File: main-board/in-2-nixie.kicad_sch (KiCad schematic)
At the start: 33 parts, among them J1 Encoder, J2 Matrix, J3 Buttons, J4 Power, J5 BME280, J6 DS3231, Q1 MPSA42, T1 IN-2, T2 IN-2, T3 IN-2, T4 IN-2, U1 HV5222PJ, U2 Nixie HVPS, U3 ESP32-C6 SuperMini, U4 Level Shifter

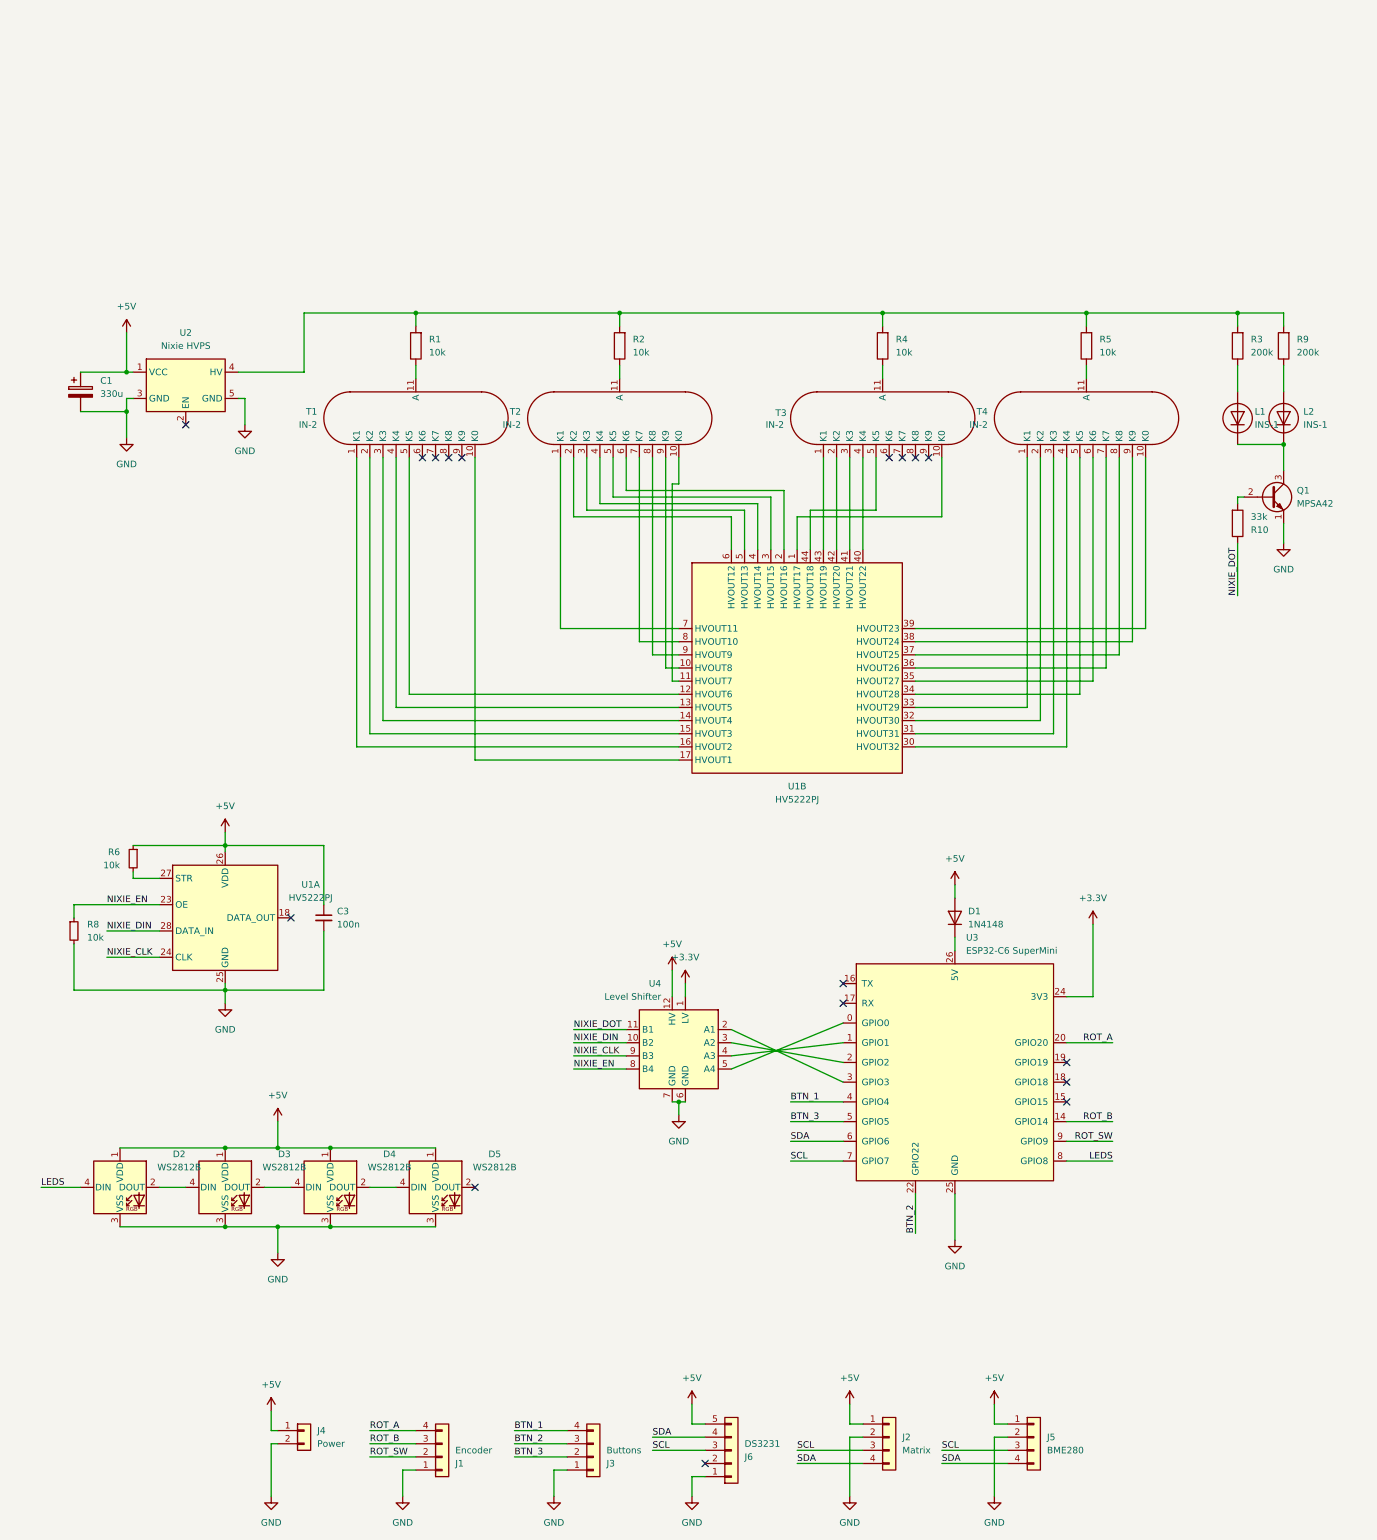
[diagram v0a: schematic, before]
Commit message: pcb final
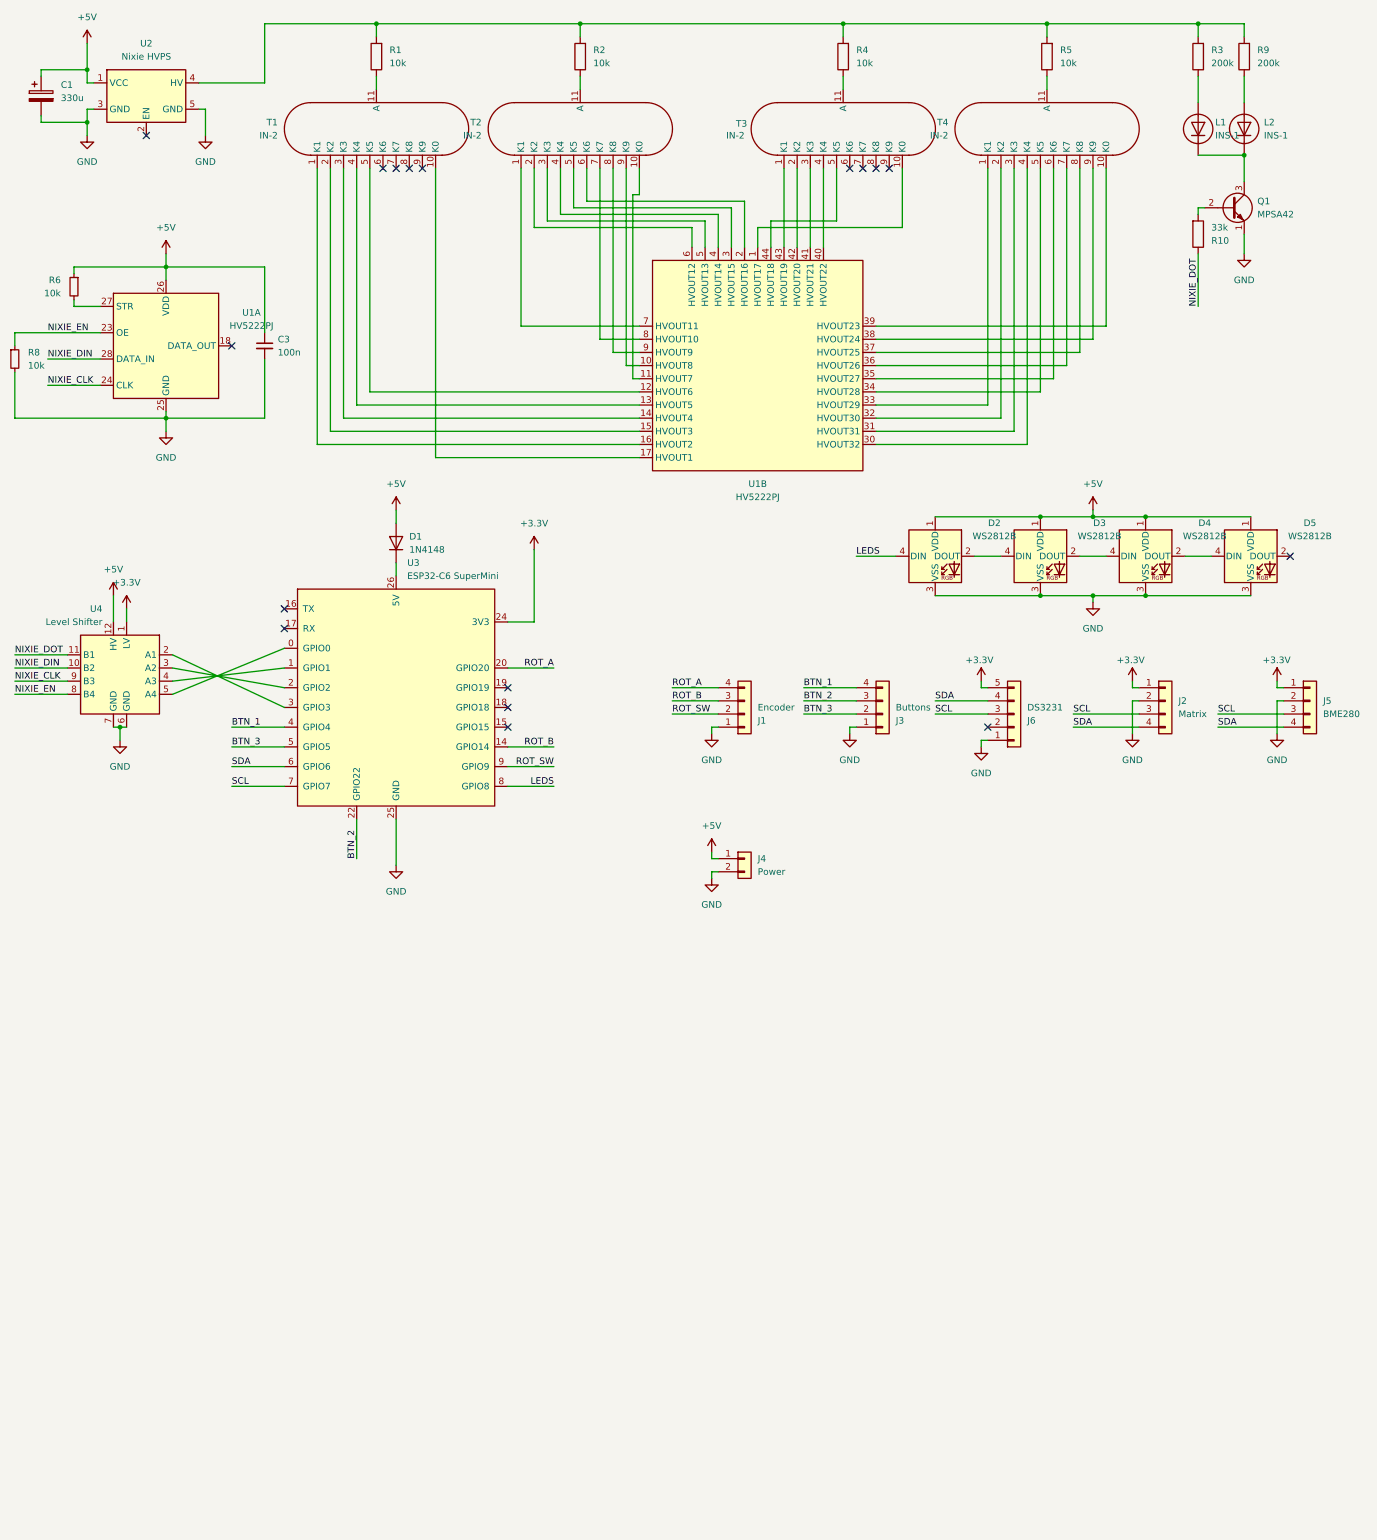
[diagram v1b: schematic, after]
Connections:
- net +3.3V: now also J2.1 (Pin_1), J5.1 (Pin_1), J6.5 (Pin_5)
- net +5V: no longer J2.1 (Pin_1), J5.1 (Pin_1), J6.5 (Pin_5)
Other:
- moved on the sheet: C1, C3, D1, D2, D3, D4, D5, J1, J2, J3, J4, J5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
